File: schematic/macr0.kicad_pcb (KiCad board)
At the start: 2 copper layers, 43.2 x 43.2 mm, 25 parts, among them J1 USB-C, J2 ISP, U1 ATmega32U4, U2 CAT4104, Y1 16MHz

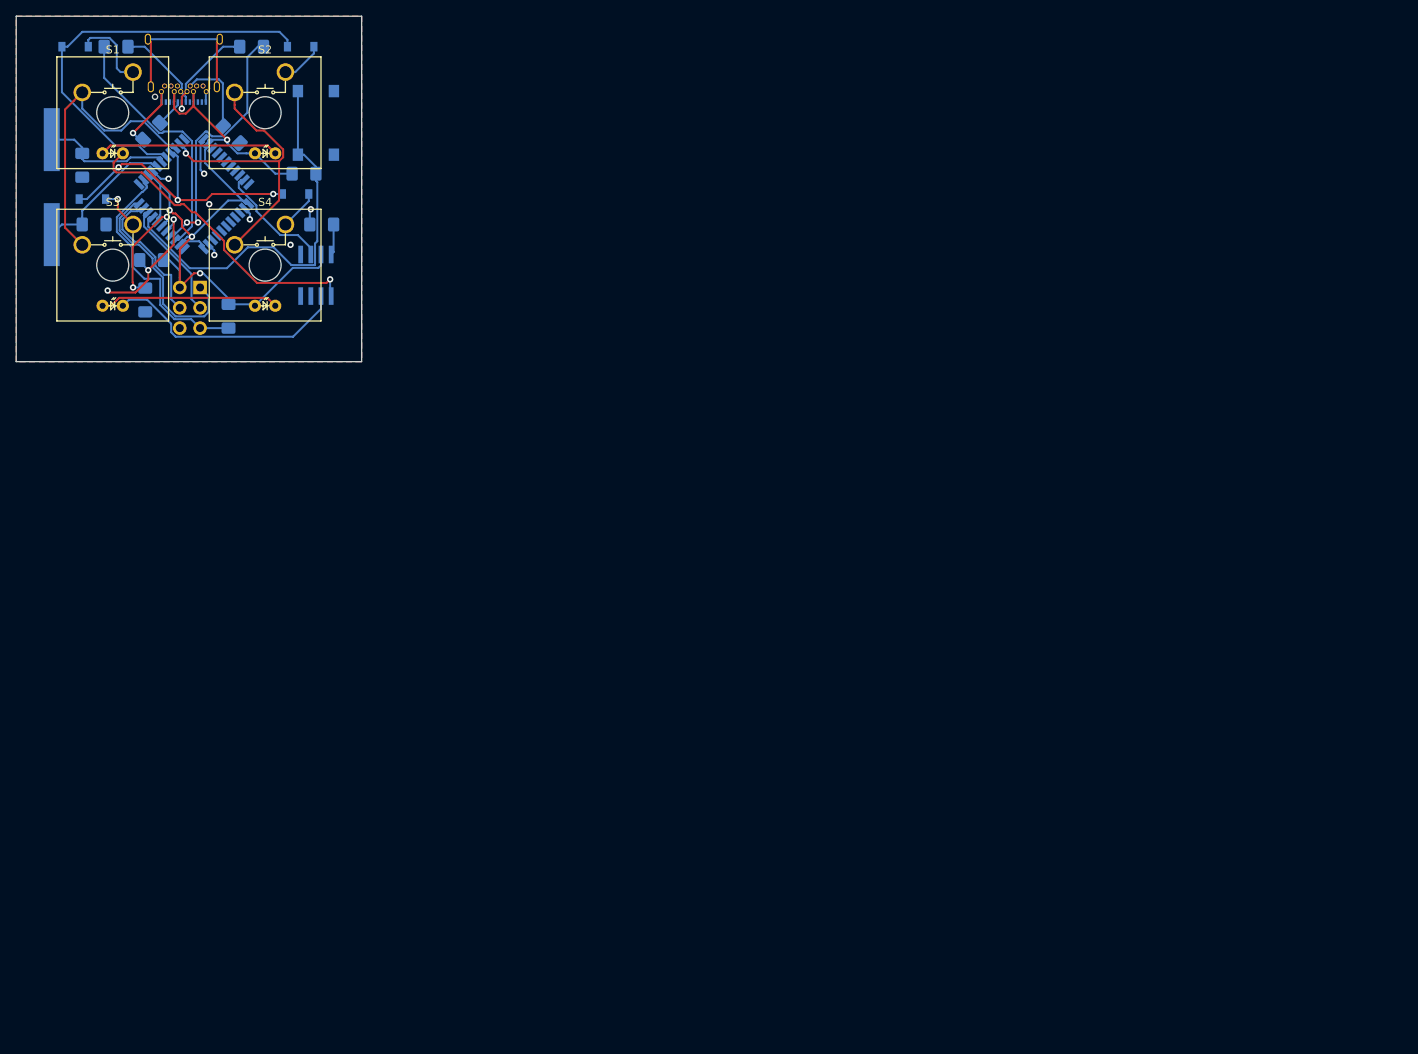
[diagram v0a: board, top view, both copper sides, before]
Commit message: First prototype pcb for fab.
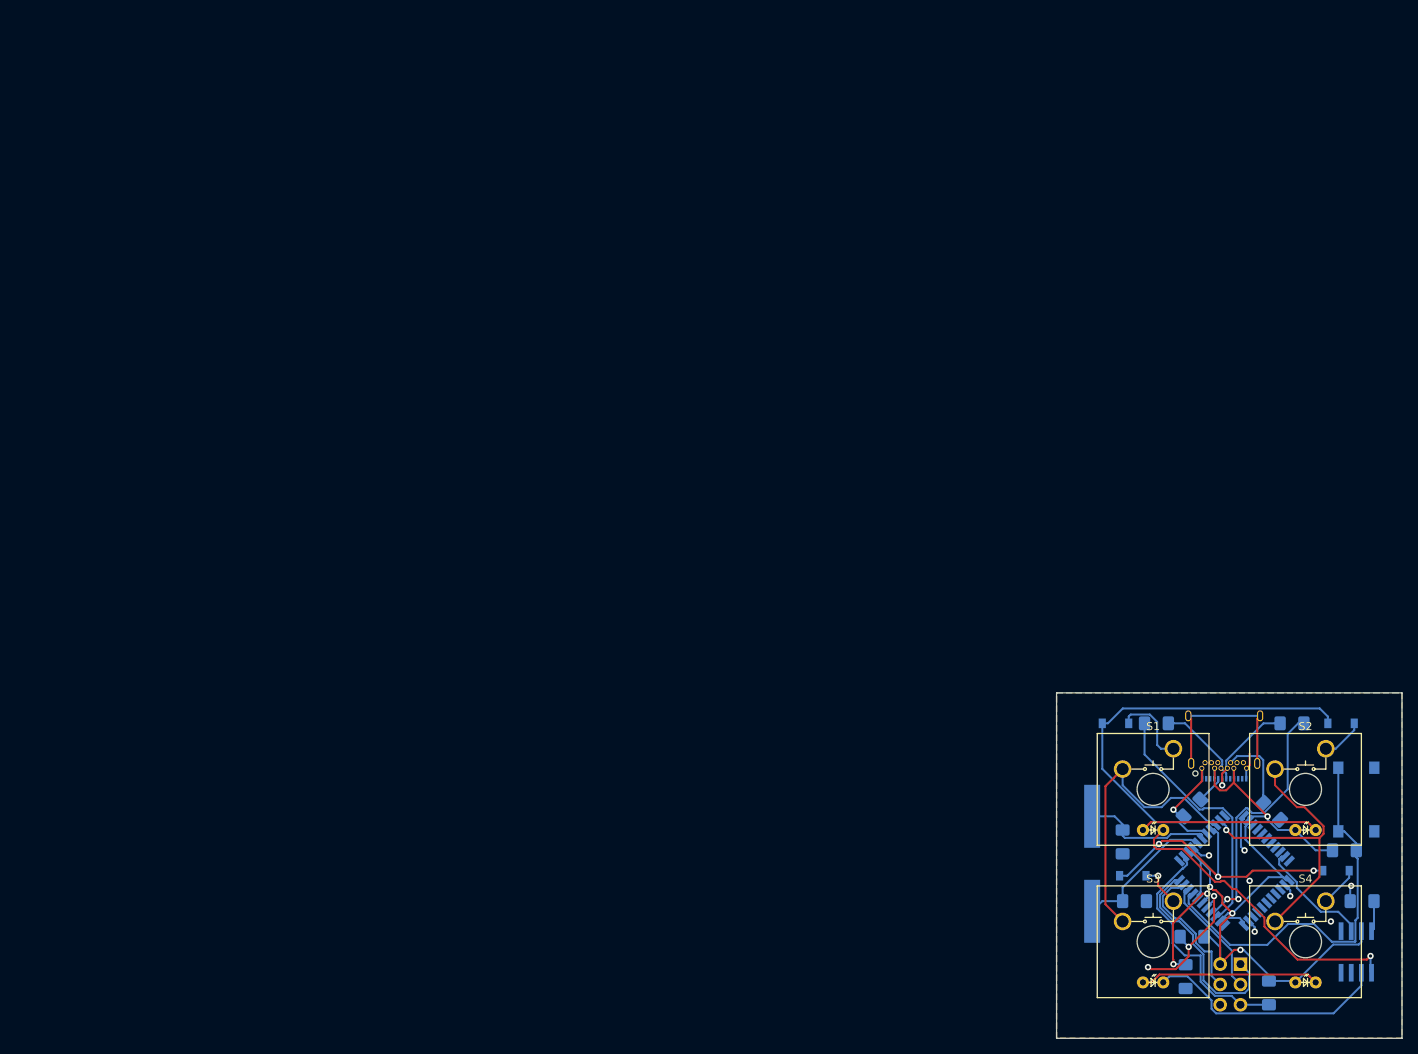
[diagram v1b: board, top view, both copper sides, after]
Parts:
- moved C1 155.1 mm to (123.7, 96.2)
- moved C2 155.1 mm to (125.2, 103.6)
- moved C3 155.1 mm to (131.6, 113.1)
- moved C4 155.1 mm to (132.4, 108.1)
- moved D1 155.1 mm to (122.8, 81.4)
- moved D2 155.1 mm to (151.0, 81.4)
- moved D3 155.1 mm to (125.0, 100.5)
- moved D4 155.1 mm to (150.4, 99.8)
- moved J1 155.1 mm to (136.4, 83.3)
- moved J2 155.1 mm to (138.4, 111.5)
- moved R1 155.1 mm to (142.0, 115.1)
- moved R2 155.1 mm to (151.4, 97.3)
- moved R3 155.1 mm to (132.4, 92.0)
- moved R4 155.1 mm to (142.3, 92.4)
- moved R5 155.1 mm to (127.9, 81.4)
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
